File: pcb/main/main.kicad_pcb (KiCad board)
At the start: 2 copper layers, 175.3 x 107.3 mm, 74 parts, among them J1 RJ45, J10 SWD, J2 USB_B, J3 BOOT1, J5 ROW0, J6 ROW1, J7 ROW2, J8 ROW3, J9 BOOT0, Q1 Q_PMOS_GDS, SW1 RST, SW10 K41, SW15 K42, SW20 K43, SW5 K40, U1 STM32F103C8T6, U2 ADNS-9800, U3 LM1084-3.3, Y1 32.768kHz, Y2 8M

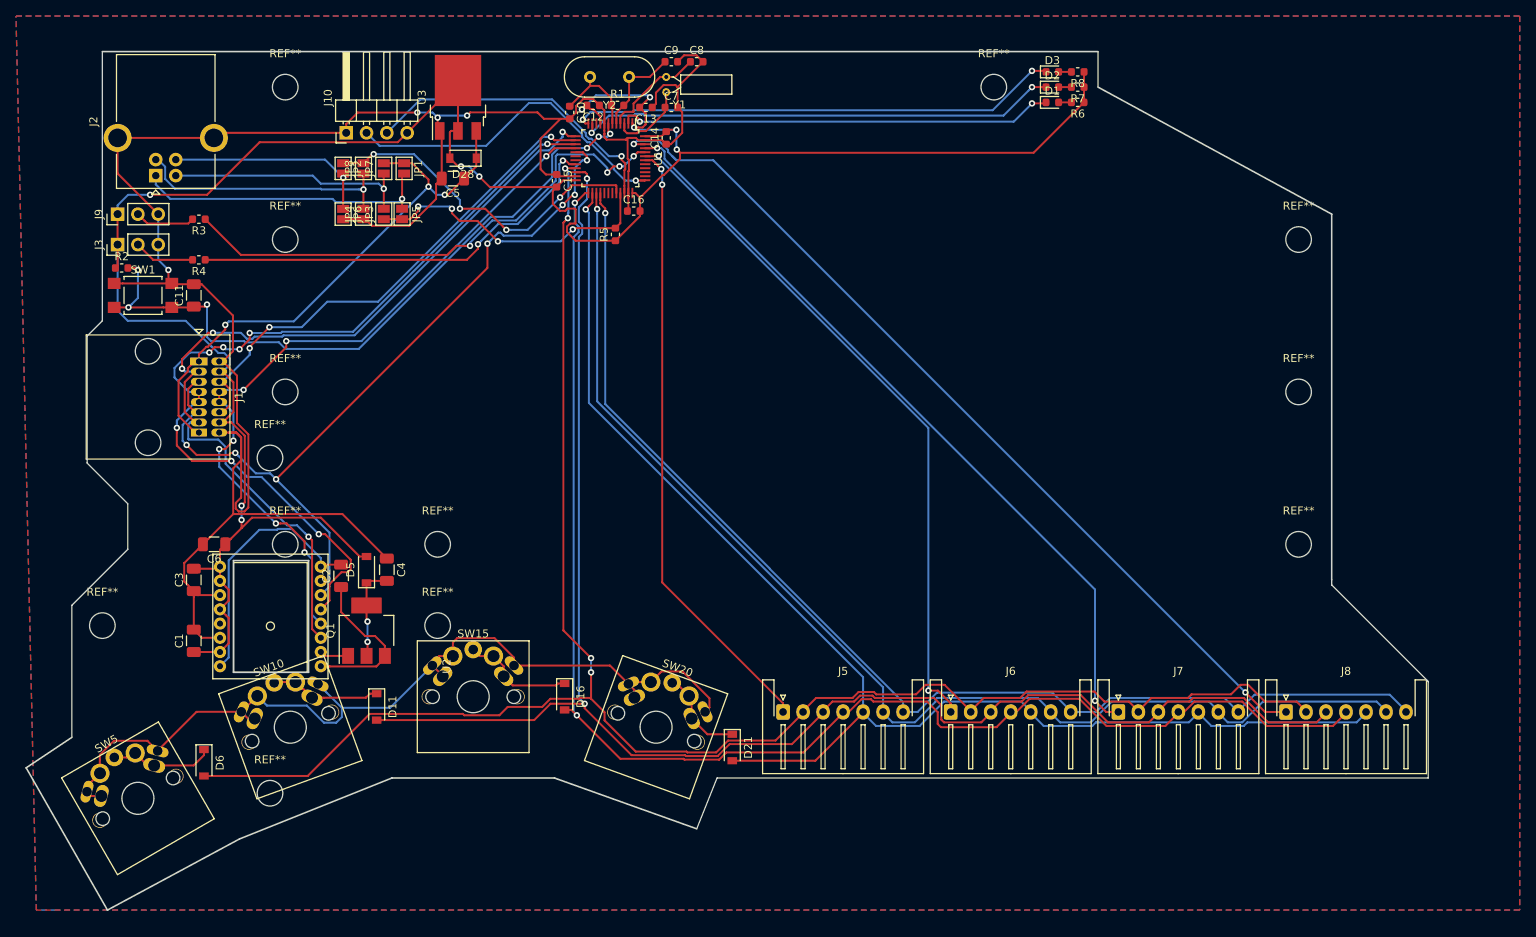
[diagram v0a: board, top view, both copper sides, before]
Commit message: revise main pcb
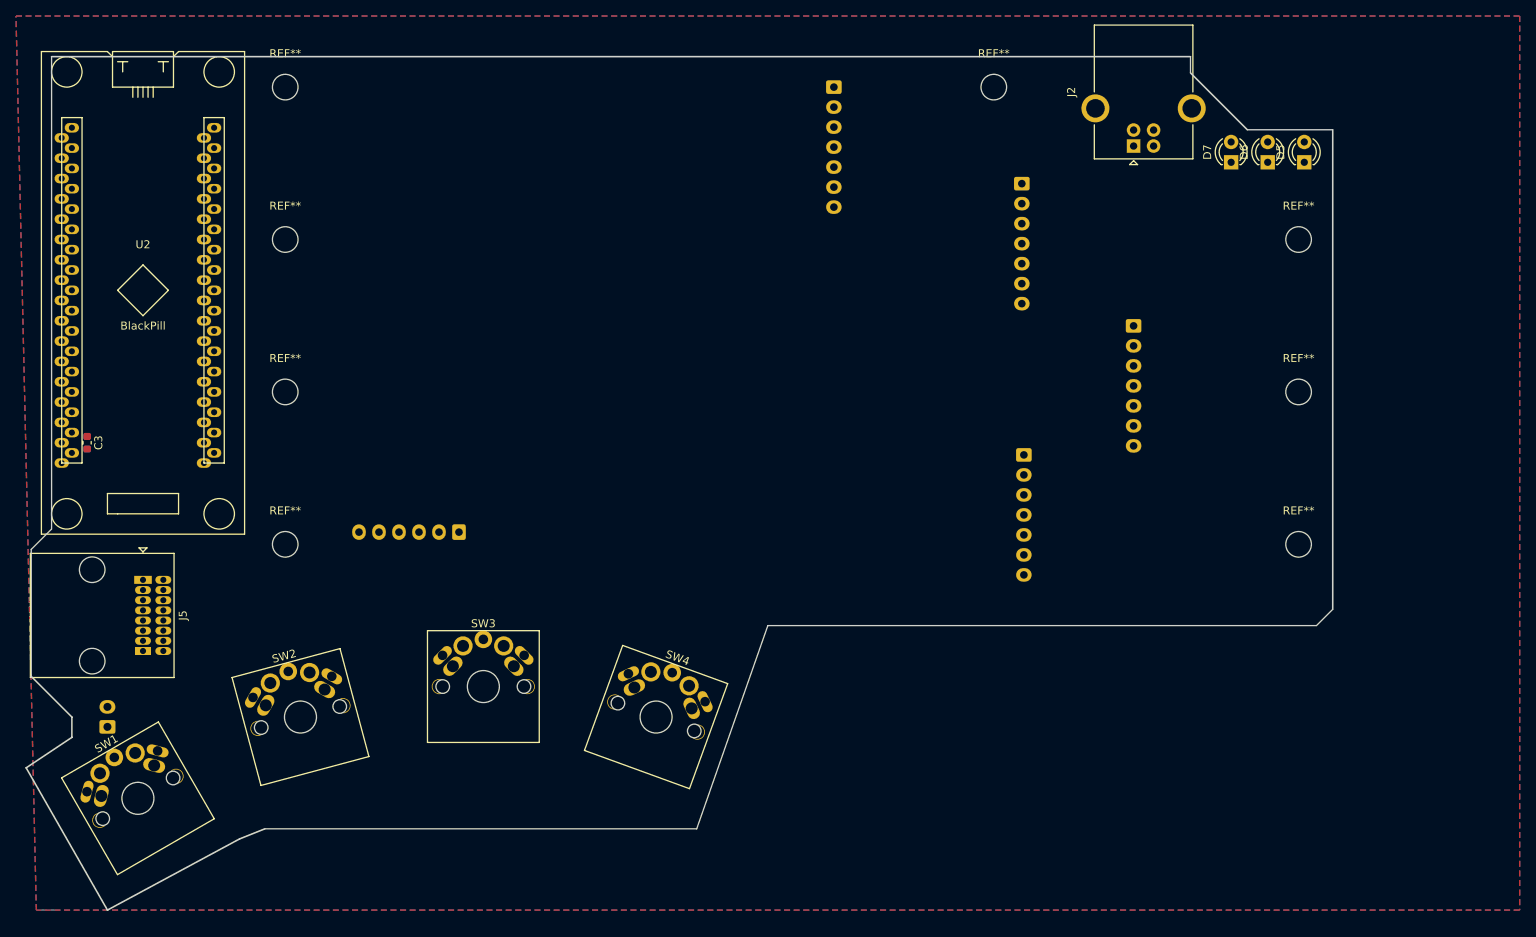
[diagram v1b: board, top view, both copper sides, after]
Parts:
- removed C1, C4, C5, C6: 10uF, Capacitor_SMD:C_1206_3216Metric
- removed C10, C9: 20pF, Capacitor_SMD:C_0603_1608Metric
- removed C11: 1uF, Capacitor_SMD:C_1206_3216Metric
- removed C12, C13, C14, C15, C16: 0.1uF, Capacitor_SMD:C_0603_1608Metric
- removed C2: 470pF, Capacitor_SMD:C_1206_3216Metric
- removed C7, C8: 12.5pF, Capacitor_SMD:C_0603_1608Metric
- removed D1, D2, D3: LED, LED_SMD:LED_0603_1608Metric
- removed D11, D16, D21, D28: D, Diode_SMD:D_SOD-123
- removed J1: RJ45, folivora:RJ45_rev
- removed J10: SWD, Connector_PinHeader_2.54mm:PinHeader_1x04_P2.54mm_Horizontal
- removed J9: BOOT0, Connector_PinHeader_2.54mm:PinHeader_1x03_P2.54mm_Vertical
- removed JP2, JP3, JP4: L, Jumper:SolderJumper-2_P1.3mm_Open_Pad1.0x1.5mm
- removed JP5, JP6, JP7, JP8: R, Jumper:SolderJumper-2_P1.3mm_Open_Pad1.0x1.5mm
- removed Q1: Q_PMOS_GDS, Package_TO_SOT_SMD:SOT-223-3_TabPin2
- removed R1: 10Mohm, Resistor_SMD:R_0603_1608Metric
- removed R2: 4.7kohm, Resistor_SMD:R_0603_1608Metric
- removed R3, R4: 10kohm, Resistor_SMD:R_0603_1608Metric
- removed R5: 1.5kohm, Resistor_SMD:R_0603_1608Metric
- removed R6, R7, R8: 140ohm, Resistor_SMD:R_0603_1608Metric
- removed the REF** at (151.8, 157.5)
- removed the REF** at (130.8, 136.5)
- removed the REF** at (109.9, 157.5)
- removed the REF** at (130.8, 178.4)
- removed the REF** at (151.8, 147.3)
- removed SW10: K41, folivora:SW_Cherry_MX1A_1.00u_PCB
- removed SW15: K42, folivora:SW_Cherry_MX1A_1.00u_PCB
- removed SW20: K43, folivora:SW_Cherry_MX1A_1.00u_PCB
- removed SW5: K40, folivora:SW_Cherry_MX1A_1.00u_PCB
- removed U1: STM32F103C8T6, Package_QFP:LQFP-48_7x7mm_P0.5mm
- removed U3: LM1084-3.3, Package_TO_SOT_SMD:TO-252-3_TabPin2
- removed Y1: 32.768kHz, Crystal:Crystal_DS26_D2.0mm_L6.0mm_Horizontal
- removed Y2: 8M, Crystal:Crystal_HC49-U_Vertical
- added D7: LED, LED_THT:LED_D3.0mm, F.Cu at (251.0, 99.6)
- added J4: ROW0, Connector_JST:JST_XH_S07B-XH-A_1x07_P2.50mm_Horizontal, B.Cu at (201.3, 90.2)
- added SW2: SW41, folivora:SW_Cherry_MX1A_1.00u_PCB, F.Cu at (134.6, 168.9)
- added SW3: SW42, folivora:SW_Cherry_MX1A_1.00u_PCB, F.Cu at (157.5, 165.1)
- added SW4: SW43, folivora:SW_Cherry_MX1A_1.00u_PCB, F.Cu at (179.1, 168.9)
- C3: value 10uF -> 0.1uF; footprint Capacitor_SMD:C_1206_3216Metric -> Capacitor_SMD:C_0603_1608Metric
- D5, D6: value D -> LED; footprint Diode_SMD:D_SOD-123 -> LED_THT:LED_D3.0mm
- J3: value BOOT1 -> Trackball_conn; footprint Connector_PinHeader_2.54mm:PinHeader_1x03_P2.54mm_Vertical -> Connector_JST:JST_XH_S06B-XH-A_1x06_P2.50mm_Horizontal; moved to B.Cu
- J5: value ROW0 -> RJ45; footprint Connector_JST:JST_XH_S07B-XH-A-1_1x07_P2.50mm_Horizontal -> folivora:RJ45_rev
- J6, J7, J8: footprint Connector_JST:JST_XH_S07B-XH-A-1_1x07_P2.50mm_Horizontal -> Connector_JST:JST_XH_S07B-XH-A_1x07_P2.50mm_Horizontal; moved to B.Cu
- JP1: value L -> slave; footprint Jumper:SolderJumper-2_P1.3mm_Open_Pad1.0x1.5mm -> Connector_JST:JST_XH_S02B-XH-A_1x02_P2.50mm_Horizontal; moved to B.Cu
- SW1: value RST -> SW40; footprint Button_Switch_SMD:SW_SPST_TL3305A -> folivora:SW_Cherry_MX1A_1.00u_PCB
- U2: value ADNS-9800 -> BlackPill; footprint folivora:ADNS-9800 -> folivora:BlackPill
- moved D6 152.7 mm to (255.5, 99.6), turned to 90 degrees
- moved D5 127.8 mm to (260.1, 99.6)
- moved J2 122.3 mm to (238.8, 97.5)
- moved J5 81.7 mm to (114.9, 151.8), turned to 270 degrees
- moved JP1 79.0 mm to (110.5, 170.1), turned to 90 degrees
- moved U2 74.2 mm to (106.0, 95.2), turned to 0 degrees
- moved J6 66.6 mm to (224.8, 102.2), turned to 270 degrees
- moved SW1 62.9 mm to (114.3, 179.1), turned to 30 degrees
- moved J3 55.8 mm to (154.4, 145.8), turned to 180 degrees
- moved J7 48.3 mm to (238.8, 120.0), turned to 270 degrees
- moved J8 45.9 mm to (225.0, 136.1), turned to 270 degrees
- moved C3 21.7 mm to (108.0, 134.6), turned to 270 degrees
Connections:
- C3 pad 1: GND -> +3V3
- C3 pad 2: +3V3 -> GND
- D5 pad 1: Net-(C4-Pad2) -> GND
- D5 pad 2: +3V3 -> Net-(D5-Pad2)
- D6 pad 1: Net-(D6-Pad1) -> GND
- D6 pad 2: /COL0 -> Net-(D6-Pad2)
- J2 pad 1: /USB_1 -> +5V
- J2 pad 2: /USB_2 -> /D-
- J2 pad 3: /USB_3 -> /D+
- J2 pad 4: /USB_4 -> GND
- J3 pad 2: /BOOT1 -> /SS_T
- J3 pad 3: GND -> /SCK
- J5 pad 1: /ROW0 -> GND
- J5 pad 2: /COL0 -> Net-(J5-Pad2)
- J5 pad 3: /COL1 -> /SCK
- J5 pad 4: /COL2 -> /MOSI
- J5 pad 5: /COL3 -> /MISO
- J5 pad 6: /COL4 -> /SS_K
- J5 pad 7: /COL5 -> /SS_T
- J6 pad 1: /ROW1 -> /SELECT1
- J6 pad 2: /COL0 -> /READ0
- J6 pad 3: /COL1 -> /READ1
- J6 pad 4: /COL2 -> /READ2
- J6 pad 5: /COL3 -> /READ3
- J6 pad 6: /COL4 -> /READ4
- J6 pad 7: /COL5 -> /READ5
- J7 pad 1: /ROW2 -> /SELECT2
- J7 pad 2: /COL0 -> /READ0
- J7 pad 3: /COL1 -> /READ1
- J7 pad 4: /COL2 -> /READ2
- J7 pad 5: /COL3 -> /READ3
- J7 pad 6: /COL4 -> /READ4
- J7 pad 7: /COL5 -> /READ5
- J8 pad 1: /ROW3 -> /SELECT3
- J8 pad 2: /COL0 -> /READ0
- J8 pad 3: /COL1 -> /READ1
- J8 pad 4: /COL2 -> /READ2
- J8 pad 5: /COL3 -> /READ3
- J8 pad 6: /COL4 -> /READ4
- J8 pad 7: /COL5 -> /READ5
- JP1 pad 1: +5V -> Net-(JP1-Pad1)
- JP1 pad 2: /USB_1 -> /SS_K
- SW1 pad 1: GND -> Net-(D1-Pad1)
- SW1 pad 2: Net-(C11-Pad1) -> /SELECT4
- U2 pad 1: Net-(C2-Pad1) -> /SELECT0
- U2 pad 10: +3V3 -> /READ0
- U2 pad 11: GND -> /READ1
- U2 pad 12: +3V3 -> /READ2
- U2 pad 13: Net-(U2-Pad13) -> /READ3
- U2 pad 14: GND -> /READ4
- U2 pad 15: +3V3 -> /READ5
- U2 pad 16: Net-(C2-Pad2) -> +3V3
- U2 pad 2: Net-(Q1-Pad1) -> /SELECT1
- U2 pad 3: /SS_Track -> /SELECT2
- U2 pad 4: /MISO -> /SELECT3
- U2 pad 5: /SCK -> /SELECT4
- U2 pad 6: /MOSI -> Net-(U2-Pad6)
- U2 pad 8: Net-(C2-Pad2) -> /D+
- U2 pad 9: +3V3 -> /D-
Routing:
- net +3V3: track 300.5 -> 0.00 mm, vias 10 -> 0
- net GND: track 280.7 -> 0.00 mm, vias 4 -> 0
- net /COL0: track 225.2 -> 0.00 mm, vias 4 -> 0
- net /COL1: track 203.3 -> 0.00 mm, vias 2 -> 0
- net /COL2: track 179.0 -> 0.00 mm, vias 2 -> 0
- net /COL3: track 167.5 -> 0.00 mm, vias 1 -> 0
- net /COL4: track 150.0 -> 0.00 mm, vias 1 -> 0
- net /COL5: track 148.9 -> 0.00 mm, vias 1 -> 0
- net /ROW3: track 113.6 -> 0.00 mm, vias 2 -> 0
- net /ROW4: track 112.3 -> 0.00 mm
- net /SCK: track 111.8 -> 0.00 mm, vias 8 -> 0
- net /SS_Track: track 111.8 -> 0.00 mm, vias 4 -> 0
- net /MOSI: track 103.3 -> 0.00 mm, vias 7 -> 0
- net /ROW2: track 97.1 -> 0.00 mm, vias 2 -> 0
- net /MISO: track 94.8 -> 0.00 mm, vias 7 -> 0
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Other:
- board size 175.3 x 107.3 mm -> 163.3 x 106.7 mm

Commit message: arrange parts
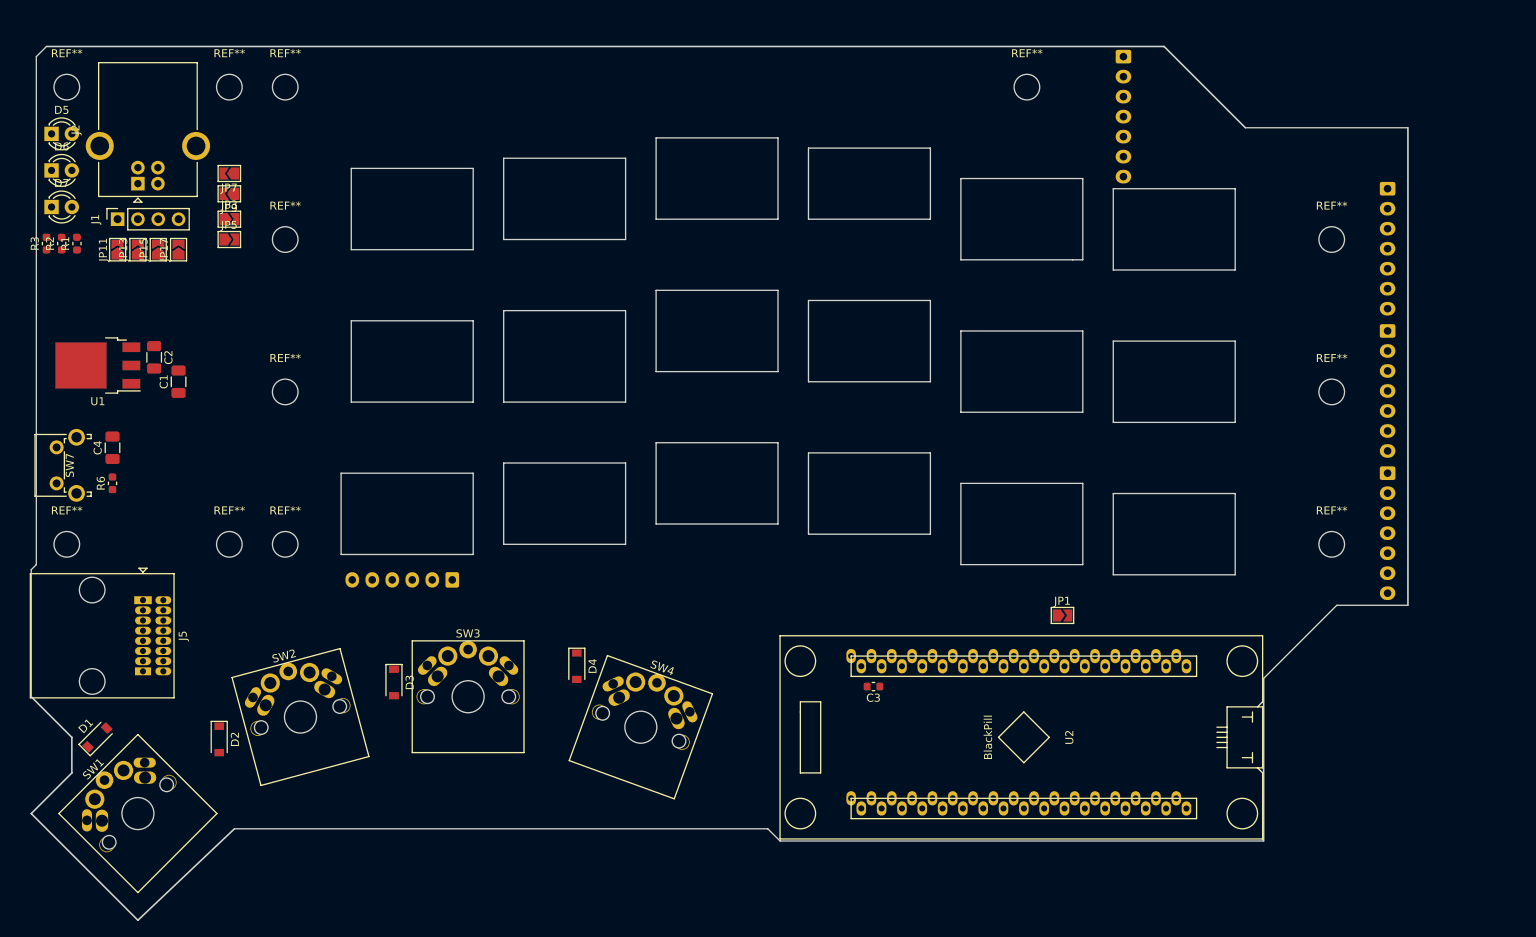
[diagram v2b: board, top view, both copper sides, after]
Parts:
- removed the REF** at (259.4, 147.3)
- removed the REF** at (259.4, 128.3)
- removed the REF** at (259.4, 109.2)
- added C1: 10uF, Capacitor_SMD:C_1206_3216Metric, F.Cu at (119.4, 127.0)
- added C2: 10uF, Capacitor_SMD:C_1206_3216Metric, F.Cu at (116.3, 124.0)
- added C4: 10uF, Capacitor_SMD:C_1206_3216Metric, F.Cu at (111.1, 135.3)
- added D1: D, Diode_SMD:D_SOD-123, F.Cu at (109.2, 171.4)
- added D2: D, Diode_SMD:D_SOD-123, F.Cu at (124.5, 171.7)
- added D3: D, Diode_SMD:D_SOD-123, F.Cu at (146.3, 164.6)
- added D4: D, Diode_SMD:D_SOD-123, F.Cu at (169.2, 162.6)
- added J1: Conn_01x04, Connector_PinSocket_2.54mm:PinSocket_1x04_P2.54mm_Vertical, F.Cu at (111.8, 106.7)
- added JP10: R, Jumper:SolderJumper-2_P1.3mm_Open_TrianglePad1.0x1.5mm, B.Cu at (111.8, 110.5)
- added JP11: L, Jumper:SolderJumper-2_P1.3mm_Open_TrianglePad1.0x1.5mm, F.Cu at (111.8, 110.5)
- added JP12: R, Jumper:SolderJumper-2_P1.3mm_Open_TrianglePad1.0x1.5mm, B.Cu at (114.3, 110.5)
- added JP13: L, Jumper:SolderJumper-2_P1.3mm_Open_TrianglePad1.0x1.5mm, F.Cu at (114.3, 110.5)
- added JP14: R, Jumper:SolderJumper-2_P1.3mm_Open_TrianglePad1.0x1.5mm, B.Cu at (116.8, 110.5)
- added JP15: L, Jumper:SolderJumper-2_P1.3mm_Open_TrianglePad1.0x1.5mm, F.Cu at (116.8, 110.5)
- added JP16: R, Jumper:SolderJumper-2_P1.3mm_Open_TrianglePad1.0x1.5mm, B.Cu at (119.4, 110.5)
- added JP17: L, Jumper:SolderJumper-2_P1.3mm_Open_TrianglePad1.0x1.5mm, F.Cu at (119.4, 110.5)
- added JP2: L, Jumper:SolderJumper-2_P1.3mm_Open_TrianglePad1.0x1.5mm, B.Cu at (125.7, 109.2)
- added JP3: R, Jumper:SolderJumper-2_P1.3mm_Open_TrianglePad1.0x1.5mm, F.Cu at (125.7, 106.7)
- added JP4: L, Jumper:SolderJumper-2_P1.3mm_Open_TrianglePad1.0x1.5mm, B.Cu at (125.7, 106.7)
- added JP5: R, Jumper:SolderJumper-2_P1.3mm_Open_TrianglePad1.0x1.5mm, F.Cu at (125.7, 109.2)
- added JP6: L, Jumper:SolderJumper-2_P1.3mm_Open_TrianglePad1.0x1.5mm, B.Cu at (125.7, 103.5)
- added JP7: R, Jumper:SolderJumper-2_P1.3mm_Open_TrianglePad1.0x1.5mm, F.Cu at (125.7, 101.0)
- added JP8: L, Jumper:SolderJumper-2_P1.3mm_Open_TrianglePad1.0x1.5mm, B.Cu at (125.7, 101.0)
- added JP9: R, Jumper:SolderJumper-2_P1.3mm_Open_TrianglePad1.0x1.5mm, F.Cu at (125.7, 103.5)
- added R1: R, Resistor_SMD:R_0603_1608Metric, F.Cu at (106.7, 109.7)
- added R2: R, Resistor_SMD:R_0603_1608Metric, F.Cu at (104.8, 109.7)
- added R3: R, Resistor_SMD:R_0603_1608Metric, F.Cu at (102.9, 109.7)
- added R6: 10k, Resistor_SMD:R_0603_1608Metric, F.Cu at (111.1, 139.7)
- added REF**: MountingHole_3.2mm_M3, MountingHole:MountingHole_3.2mm_M3, F.Cu at (105.4, 90.2)
- added REF**: MountingHole_3.2mm_M3, MountingHole:MountingHole_3.2mm_M3, F.Cu at (125.7, 147.3)
- added REF**: MountingHole_3.2mm_M3, MountingHole:MountingHole_3.2mm_M3, F.Cu at (105.4, 147.3)
- added REF**: MountingHole_3.2mm_M3, MountingHole:MountingHole_3.2mm_M3, F.Cu at (263.5, 147.3)
- added REF**: MountingHole_3.2mm_M3, MountingHole:MountingHole_3.2mm_M3, F.Cu at (263.5, 128.3)
- added REF**: MountingHole_3.2mm_M3, MountingHole:MountingHole_3.2mm_M3, F.Cu at (263.5, 109.2)
- added REF**: MountingHole_3.2mm_M3, MountingHole:MountingHole_3.2mm_M3, F.Cu at (125.7, 90.2)
- added SW7: RST, Button_Switch_THT:SW_Tactile_SPST_Angled_PTS645Vx31-2LFS, F.Cu at (104.1, 139.7)
- added U1: 3.3v regul, Package_TO_SOT_SMD:TO-252-3_TabPin2, F.Cu at (109.3, 125.0)
- JP1: footprint Connector_JST:JST_XH_S02B-XH-A_1x02_P2.50mm_Horizontal -> Jumper:SolderJumper-2_P1.3mm_Open_TrianglePad1.0x1.5mm; moved to F.Cu
- moved D5 156.6 mm to (103.5, 96.0), turned to 0 degrees
- moved U2 154.7 mm to (245.4, 162.6), turned to 270 degrees
- moved D6 152.0 mm to (103.5, 100.6), turned to 0 degrees
- moved D7 147.6 mm to (103.5, 105.2), turned to 0 degrees
- moved J2 124.5 mm to (114.3, 102.2)
- moved JP1 120.2 mm to (229.9, 156.2), turned to 0 degrees
- moved C3 102.9 mm to (206.2, 165.1), turned to 180 degrees
- moved J6 45.7 mm to (270.5, 102.9)
- moved J8 45.5 mm to (270.5, 138.4)
- moved J4 36.4 mm to (237.5, 86.4)
- moved J7 31.8 mm to (270.5, 120.7)
- moved J3 6.03 mm to (153.6, 151.8)
- moved REF** 4.14 mm to (225.4, 90.2)
- moved J5 2.54 mm to (114.9, 154.3)
- moved SW3 2.29 mm to (155.6, 166.4)
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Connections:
- D5 pad 1: GND -> /LED1
- D6 pad 1: GND -> /LED2
- D7 pad 1: GND -> /LED3
- J2 pad 1: +5V -> /USB_1
- J2 pad 2: /D- -> /USB_2
- J2 pad 3: /D+ -> /USB_3
- J2 pad 4: GND -> /USB_4
- U2 pad 21: Net-(U2-Pad21) -> /RST
- U2 pad 22: Net-(U2-Pad22) -> /LED3
- U2 pad 23: Net-(U2-Pad23) -> /LED2
- U2 pad 24: Net-(U2-Pad24) -> /LED1
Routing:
- removed copper zone on B.Cu, net GND
- removed copper zone on F.Cu, net GND
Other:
- board size 163.3 x 106.7 mm -> 172.1 x 109.2 mm
